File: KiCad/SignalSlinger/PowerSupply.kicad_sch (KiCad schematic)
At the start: 31 parts, among them J201 Barrel_Jack_Switch, J202 Conn_01x03, U201 LP2985-3.3, U202 LP2985-3.3, U203 TPS63060

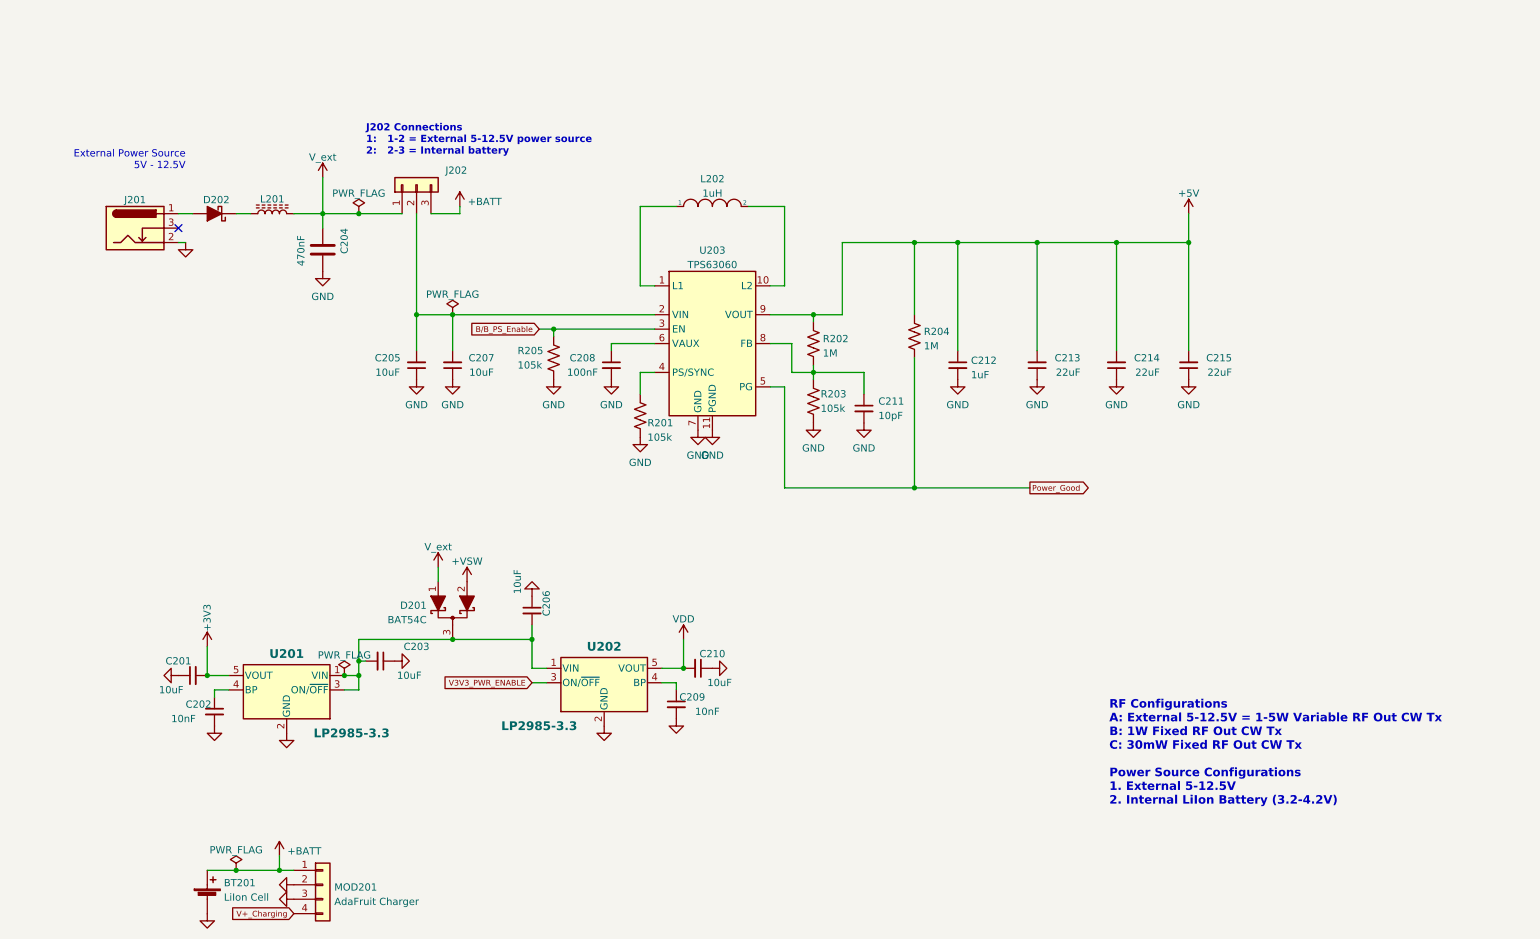
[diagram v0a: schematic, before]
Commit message: Updates
o Updated Gerbers
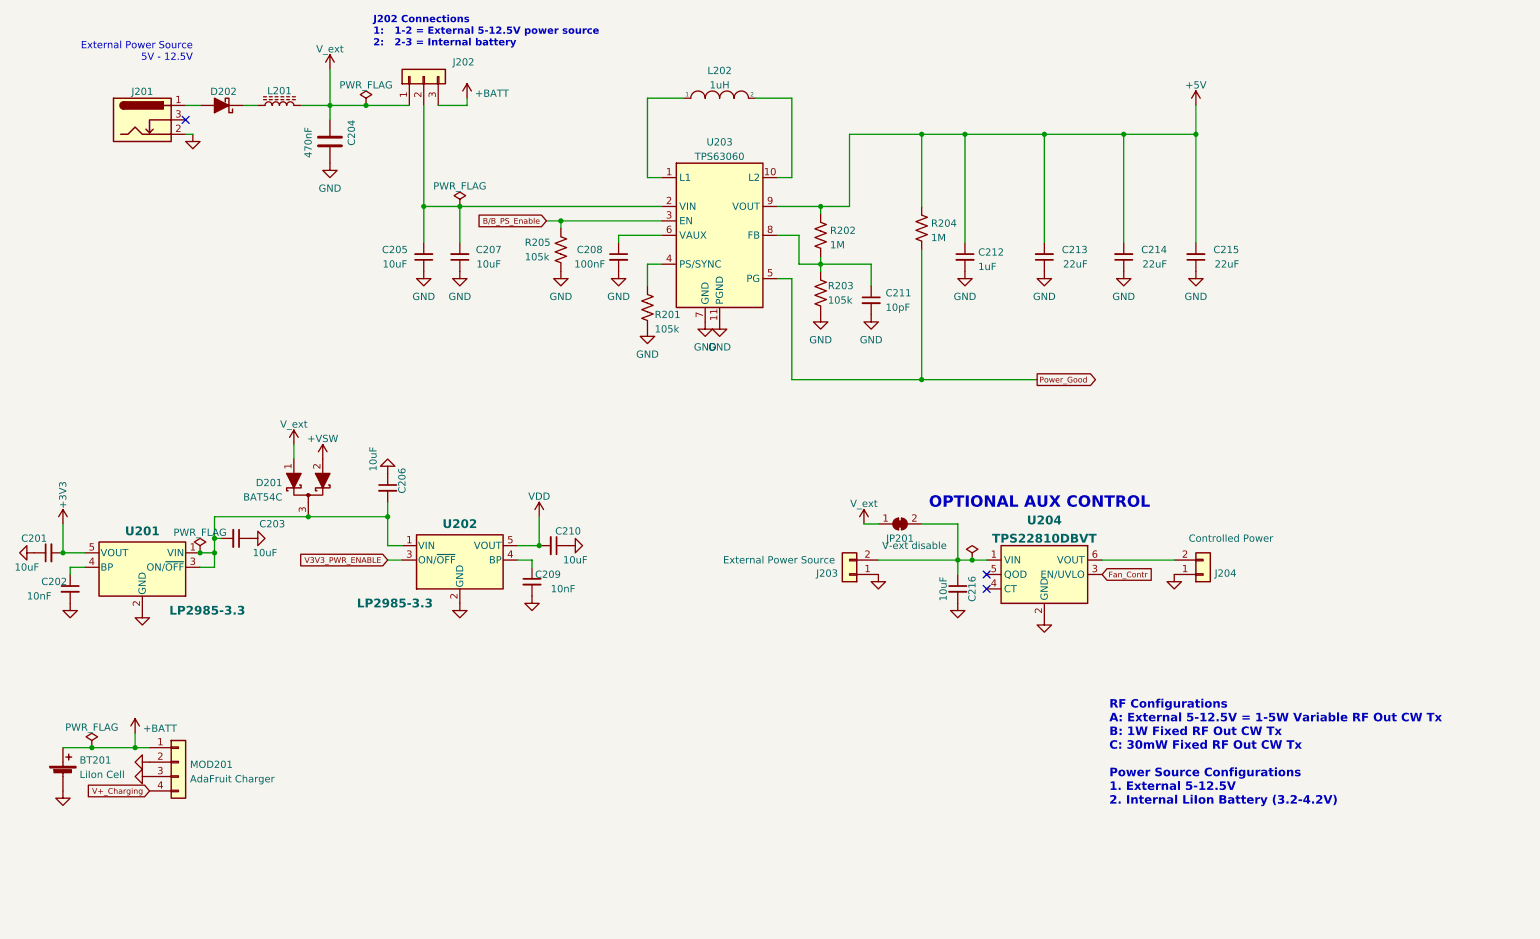
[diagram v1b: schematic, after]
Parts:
- added C216: 10uF, Capacitor_SMD:C_0805_2012Metric, symbol Device:C_Small
- added J203: External Power Source, Connector_PinHeader_2.54mm:PinHeader_1x02_P2.54mm_Vertical, symbol Connector_Generic:Conn_01x02
- added J204: Controlled Power, Connector_PinHeader_2.54mm:PinHeader_1x02_P2.54mm_Vertical, symbol Connector_Generic:Conn_01x02
- added JP201: V-ext disable, Jumper:SolderJumper-2_P1.3mm_Bridged_RoundedPad1.0x1.5mm, symbol Jumper:SolderJumper_2_Bridged
- added U204: TPS22810DBVT, Package_TO_SOT_SMD:SOT-23-6, symbol Power_Management:TPS22810DBVT
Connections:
- net GND: now also C216.2, J203.1 (Pin_1), J204.1 (Pin_1), U204.2 (GND)
- net V_ext: now also JP201.1 (A)
- new net: C216.1, J203.2 (Pin_2), JP201.2 (B), U204.1 (VIN)
- new net: J204.2 (Pin_2), U204.6 (VOUT)
- new net Fan_Contr: U204.3 (EN/UVLO)
- no-connect marks 1 -> 3
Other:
- note added: "OPTIONAL AUX CONTROL"
- moved on the sheet: BT201, C201, C202, C203, C204, C205, C206, C207, C208, C209, C210, C211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
